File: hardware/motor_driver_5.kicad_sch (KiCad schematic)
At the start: 15 parts, among them J4 B2B-XH-A(LF)(SN), U3 DRV8701ERGET, U4 DMHT6016LFJ-13

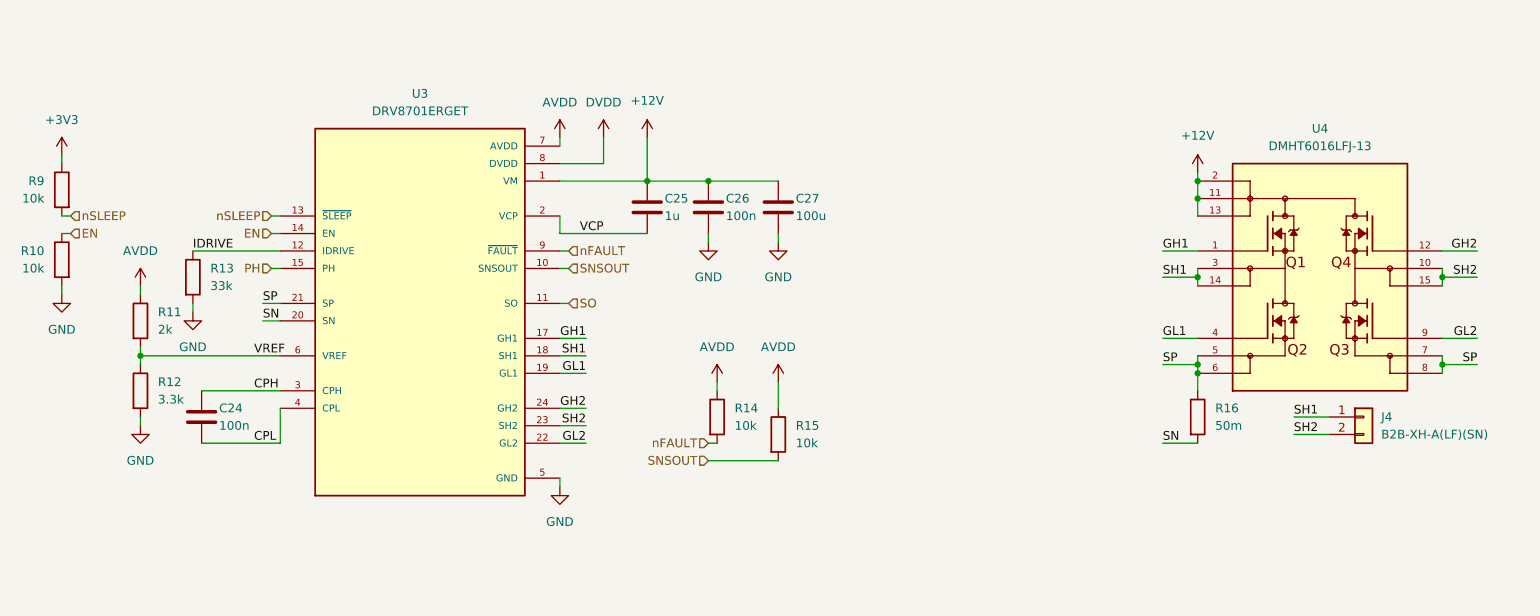
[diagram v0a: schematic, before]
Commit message: Organize schematic
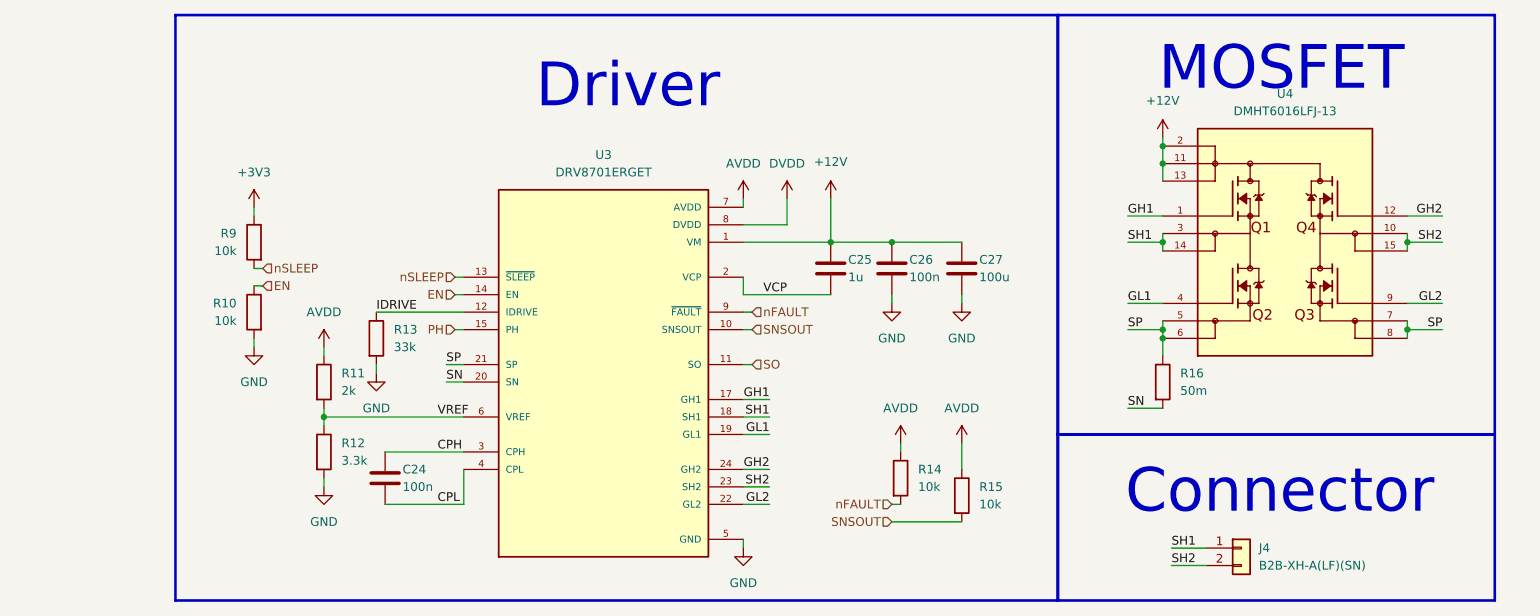
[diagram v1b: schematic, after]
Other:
- note added: "Connector"
- note added: "Driver"
- note added: "MOSFET"
- moved on the sheet: C24, C25, C26, C27, J4, R10, R11, R12, R13, R14, R15, R16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
